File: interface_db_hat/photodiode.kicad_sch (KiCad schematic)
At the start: 28 parts, among them J7 USB_B_Mini, U3 ADS1115IDGS, U4 OPA320AIDBVR, U5 OPA320AIDBVR, U6 TMUX1209PWR

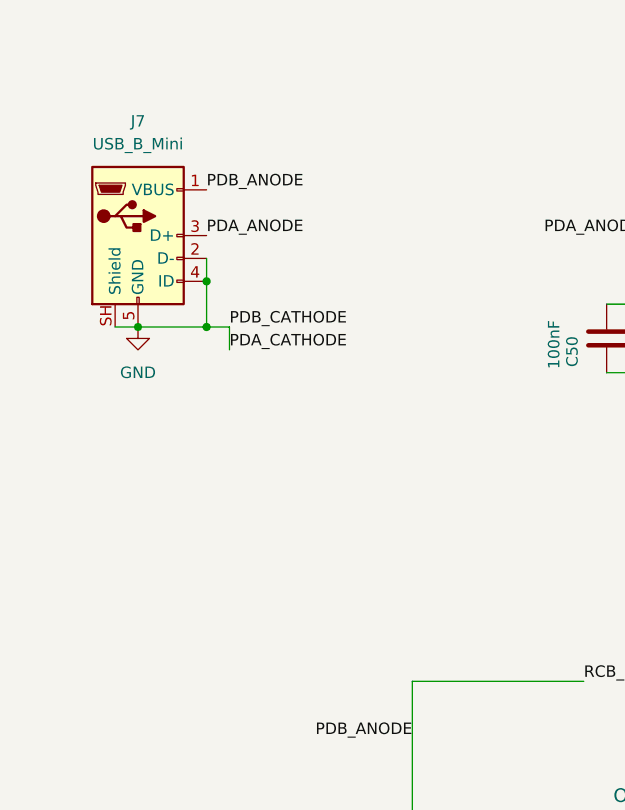
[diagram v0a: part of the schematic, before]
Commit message: update
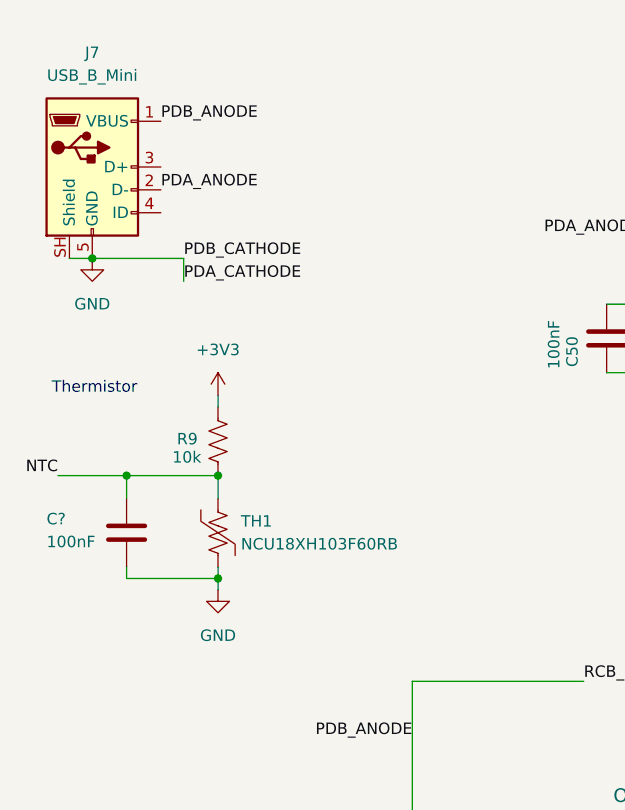
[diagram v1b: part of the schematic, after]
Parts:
- added C?: 100nF, Capacitor_SMD:C_0603_1608Metric, symbol Device:C
- added R9: 10k, Resistor_SMD:R_0603_1608Metric, symbol Device:R_US
- added TH1: NCU18XH103F60RB, Resistor_SMD:R_0603_1608Metric, symbol Device:Thermistor_US
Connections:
- net GND: now also C?.2, TH1.2; no longer J7.2 (D-), J7.4 (ID)
- net PDA_ANODE: now also J7.2 (D-); no longer J7.3 (D+)
- new net +3V3: R9.2
- new net NTC: C?.1, R9.1, TH1.1
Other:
- note added: "Thermistor"
- moved on the sheet: J7

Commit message: jlc order
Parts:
- removed C50, C51, C52: 100nF, Capacitor_SMD:C_0603_1608Metric_Pad1.08x0.95mm_HandSolder, symbol Device:C
- removed C54, C58: 1nF, Capacitor_SMD:C_0603_1608Metric_Pad1.08x0.95mm_HandSolder, symbol Device:C
- removed C55, C59: 330pF, Capacitor_SMD:C_0603_1608Metric_Pad1.08x0.95mm_HandSolder, symbol Device:C
- removed C56, C60: 100pF, Capacitor_SMD:C_0603_1608Metric_Pad1.08x0.95mm_HandSolder, symbol Device:C
- removed C57, C61: 33pF, Capacitor_SMD:C_0603_1608Metric_Pad1.08x0.95mm_HandSolder, symbol Device:C
- removed C?: 100nF, Capacitor_SMD:C_0603_1608Metric, symbol Device:C
- removed J7: USB_B_Mini, Connector_USB:USB_Mini-B_Wuerth_65100516121_Horizontal, symbol Connector:USB_B_Mini
- removed JP9: SolderJumper_2_Open, Jumper:SolderJumper-2_P1.3mm_Open_TrianglePad1.0x1.5mm, symbol Jumper:SolderJumper_2_Open
- removed R20: 50, Resistor_SMD:R_0603_1608Metric_Pad0.98x0.95mm_HandSolder, symbol Device:R_US
- removed R22, R28: 100, Resistor_SMD:R_0603_1608Metric_Pad0.98x0.95mm_HandSolder, symbol Device:R_US
- removed R23, R29: 1k, Resistor_SMD:R_0603_1608Metric_Pad0.98x0.95mm_HandSolder, symbol Device:R_US
- removed R24, R25: 0, Resistor_SMD:R_0603_1608Metric_Pad0.98x0.95mm_HandSolder, symbol Device:R_US
- removed R26, R30: 10k, Resistor_SMD:R_0603_1608Metric_Pad0.98x0.95mm_HandSolder, symbol Device:R_US
- removed R27, R31: 100k, Resistor_SMD:R_0603_1608Metric_Pad0.98x0.95mm_HandSolder, symbol Device:R_US
- removed R9: 10k, Resistor_SMD:R_0603_1608Metric, symbol Device:R_US
- removed TH1: NCU18XH103F60RB, Resistor_SMD:R_0603_1608Metric, symbol Device:Thermistor_US
- removed U3: ADS1115IDGS, Package_SO:TSSOP-10_3x3mm_P0.5mm, symbol Analog_ADC:ADS1115IDGS
- removed U4, U5: OPA320AIDBVR, OPA320:DBV5, symbol OPA320:OPA320AIDBVR
- removed U6: TMUX1209PWR, Package_SO:TSSOP-16_4.4x5mm_P0.65mm, symbol TMUX1209:TMUX1209PWR
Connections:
- no-connect marks 2 -> 0
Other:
- note removed: "Thermistor"
- note removed: "Tied to interrupt pin"
